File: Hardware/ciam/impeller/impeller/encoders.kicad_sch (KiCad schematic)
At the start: 33 parts, among them J11 Micro-Fit_2x2P, J12 Micro-Fit_2x2P, J13 Micro-Fit_2x2P, J14 Micro-Fit_2x2P, J9 Micro-Fit_2x2P, U19 TLP521-2, U4 B0505MT-1WR4

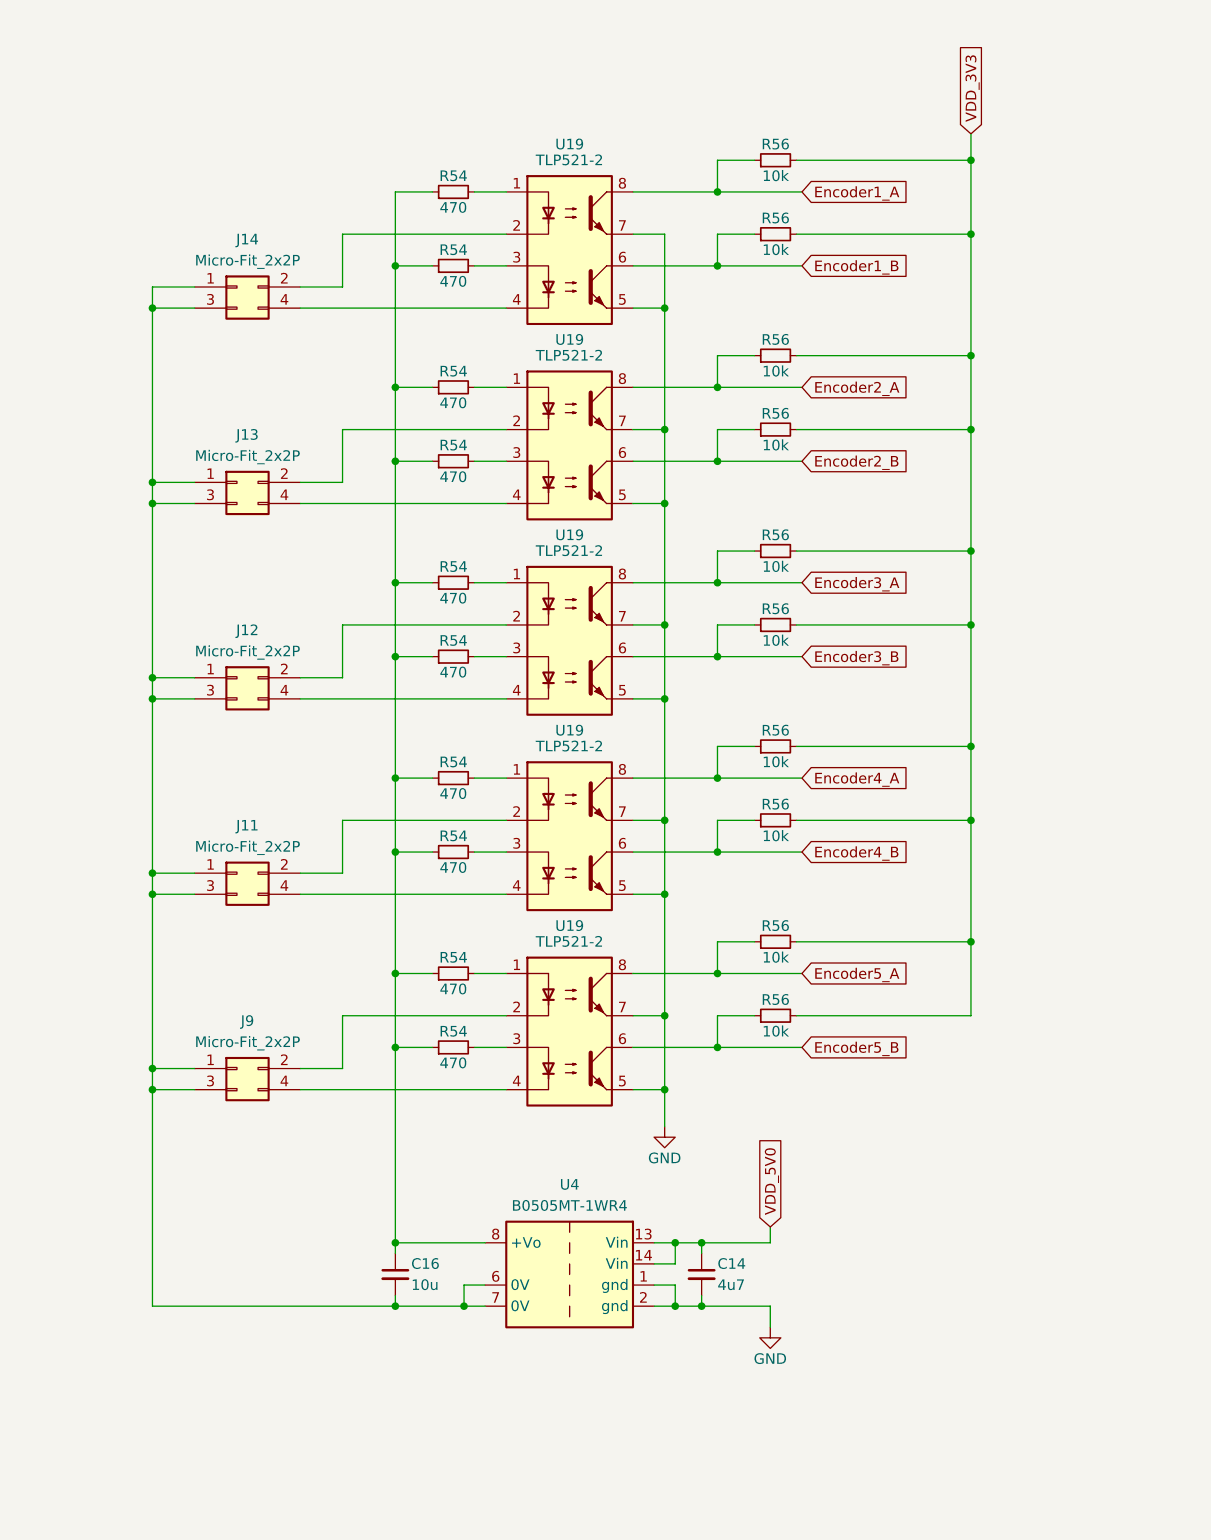
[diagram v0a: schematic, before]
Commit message: updated impeller project
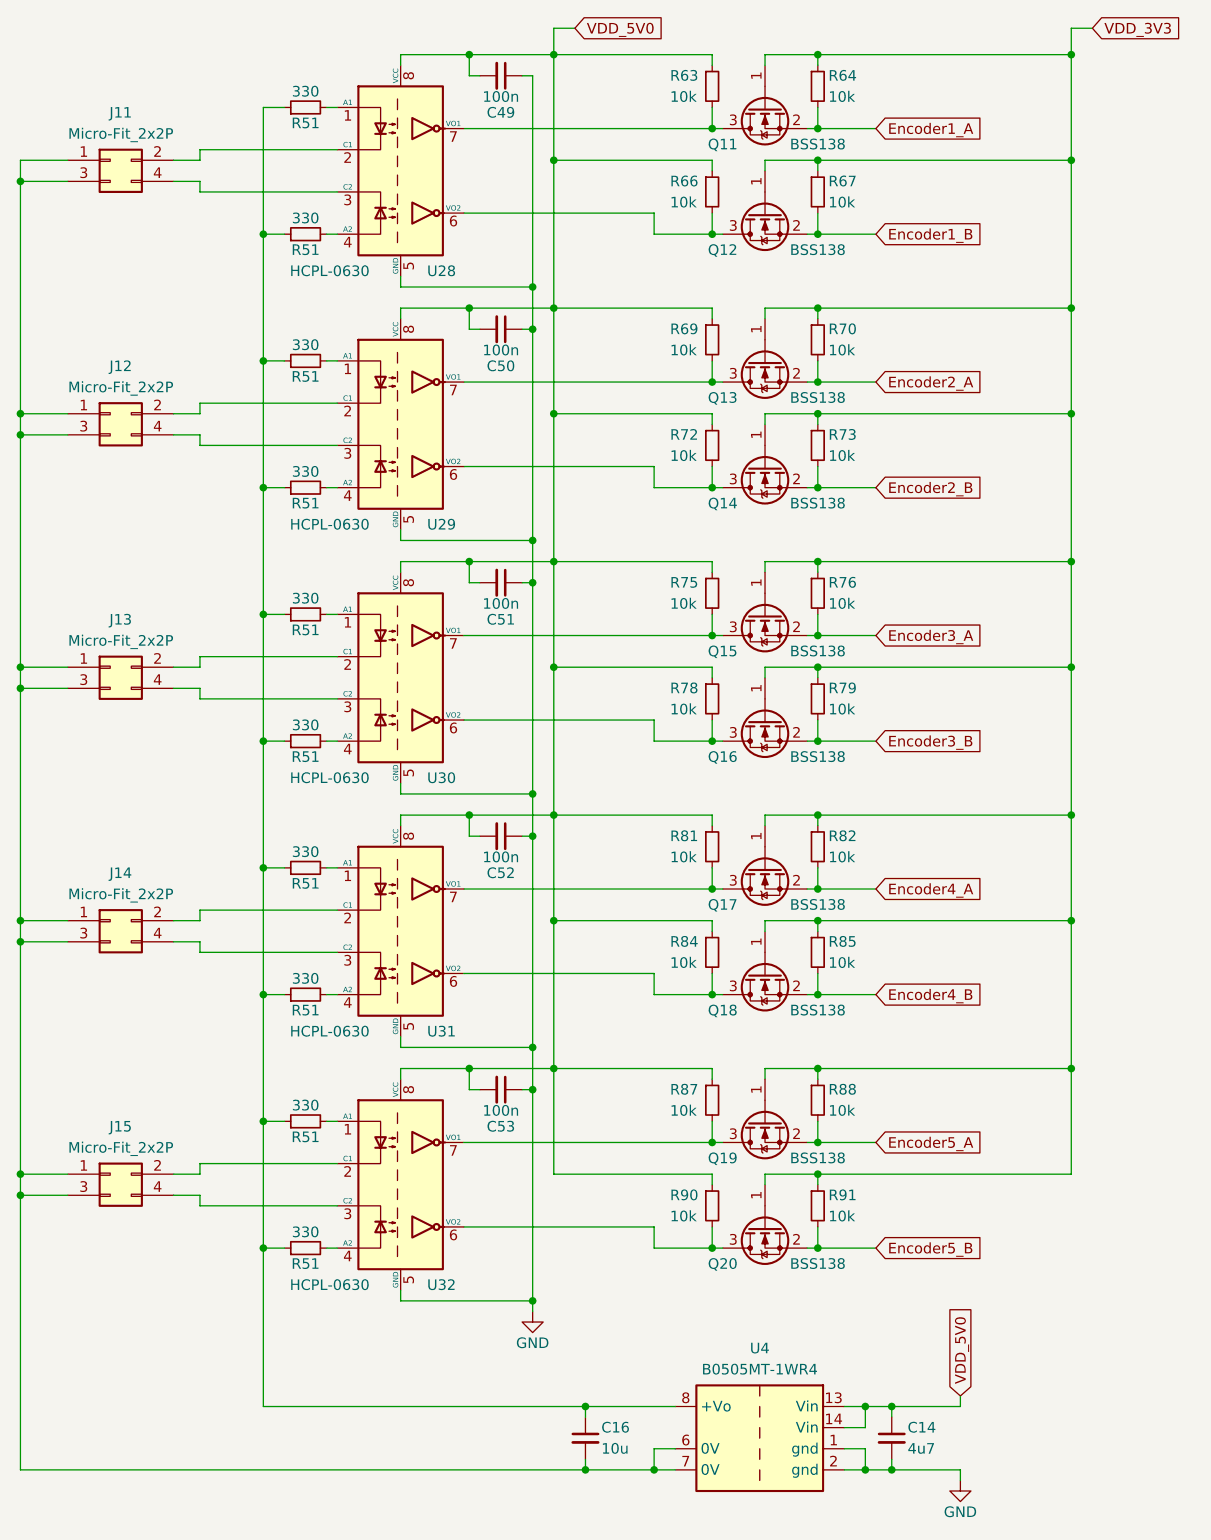
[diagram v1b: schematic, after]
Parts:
- removed R54 (x10): 470, symbol Device:R_Small
- removed R56 (x10): 10k, symbol Device:R_Small
- removed U19 (x5): TLP521-2, symbol Isolator:TLP291
- added C49, C50, C51, C52, C53: 100n, symbol Device:C_Small
- added Q11, Q12, Q13, Q14, Q15, Q16, Q17, Q18, Q19, Q20: BSS138, Package_TO_SOT_SMD:SOT-23, symbol Transistor_FET:BSS138
- added R51 (x10): 330, symbol Device:R_Small
- added R63, R64, R66, R67, R69, R70, R72, R73, R75, R76, R78, R79, R81, R82, R84, R85, R87, R88, R90, R91: 10k, symbol Device:R_Small
- added U28, U29, U30, U31, U32: HCPL-0630, Package_SO:SOIC-8_3.9x4.9mm_P1.27mm, symbol Isolator:HCPL-0630
- renumbered J9 to J15
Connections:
- net Encoder1_A: now also Q11.2 (S), R64.2
- net Encoder1_B: now also Q12.2 (S), R67.2
- net Encoder2_A: now also Q13.2 (S), R70.2
- net Encoder2_B: now also Q14.2 (S), R73.2
- net Encoder3_A: now also Q15.2 (S), R76.2
- net Encoder3_B: now also Q16.2 (S), R79.2
- net Encoder4_A: now also Q17.2 (S), R82.2
- net Encoder4_B: now also Q18.2 (S), R85.2
- net Encoder5_A: now also Q19.2 (S), R88.2
- net Encoder5_B: now also Q20.2 (S), R91.2
- net GND: now also C49.1, C50.1, C51.1, C52.1, C53.1, U28.5 (GND), U29.5 (GND), U30.5 (GND), U31.5 (GND), U32.5 (GND)
- net VDD_3V3: now also Q11.1 (G), Q12.1 (G), Q13.1 (G), Q14.1 (G), Q15.1 (G), Q16.1 (G), Q17.1 (G), Q18.1 (G), Q19.1 (G), Q20.1 (G), R64.1, R67.1, R70.1, R73.1, R76.1, R79.1, R82.1, R85.1, R88.1, R91.1
- net VDD_5V0: now also C49.2, C50.2, C51.2, C52.2, C53.2, R63.1, R66.1, R69.1, R72.1, R75.1, R78.1, R81.1, R84.1, R87.1, R90.1, U28.8 (VCC), U29.8 (VCC), U30.8 (VCC), U31.8 (VCC), U32.8 (VCC)
- net at C16.1, U4.8 (+Vo): now also R51.1, R51.1, R51.1, R51.1, R51.1, R51.1, R51.1, R51.1, R51.1, R51.1
- net at J11.2 (Pin_2): now also U28.2 (C1)
- net at J11.4 (Pin_4): now also U28.3 (C2)
- net at J15.2 (Pin_2): now also U32.2 (C1)
- net at J15.4 (Pin_4): now also U32.3 (C2)
- net at J12.2 (Pin_2): now also U29.2 (C1)
- net at J12.4 (Pin_4): now also U29.3 (C2)
- net at J13.2 (Pin_2): now also U30.2 (C1)
- net at J13.4 (Pin_4): now also U30.3 (C2)
- net at J14.2 (Pin_2): now also U31.2 (C1)
- net at J14.4 (Pin_4): now also U31.3 (C2)
- new net: R51.2, U32.1 (A1)
- new net: R51.2, U28.1 (A1)
- new net: Q11.3 (D), R63.2, U28.7 (VO1)
- new net: R51.2, U28.4 (A2)
- new net: Q12.3 (D), R66.2, U28.6 (VO2)
- new net: Q20.3 (D), R90.2, U32.6 (VO2)
- new net: R51.2, U30.1 (A1)
- new net: Q19.3 (D), R87.2, U32.7 (VO1)
- new net: Q15.3 (D), R75.2, U30.7 (VO1)
- new net: Q14.3 (D), R72.2, U29.6 (VO2)
- new net: R51.2, U31.1 (A1)
- new net: R51.2, U32.4 (A2)
- new net: Q16.3 (D), R78.2, U30.6 (VO2)
- new net: Q18.3 (D), R84.2, U31.6 (VO2)
- new net: R51.2, U31.4 (A2)
- new net: Q17.3 (D), R81.2, U31.7 (VO1)
- new net: R51.2, U29.1 (A1)
- new net: R51.2, U29.4 (A2)
- new net: Q13.3 (D), R69.2, U29.7 (VO1)
- new net: R51.2, U30.4 (A2)
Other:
- moved on the sheet: C14, C16, J15, U4
